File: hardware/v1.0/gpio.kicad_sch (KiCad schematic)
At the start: 23 parts, among them J2 HDMI_C_1.3, U1 ECP5U_12_CABGA256, U5 PCA9306DC1

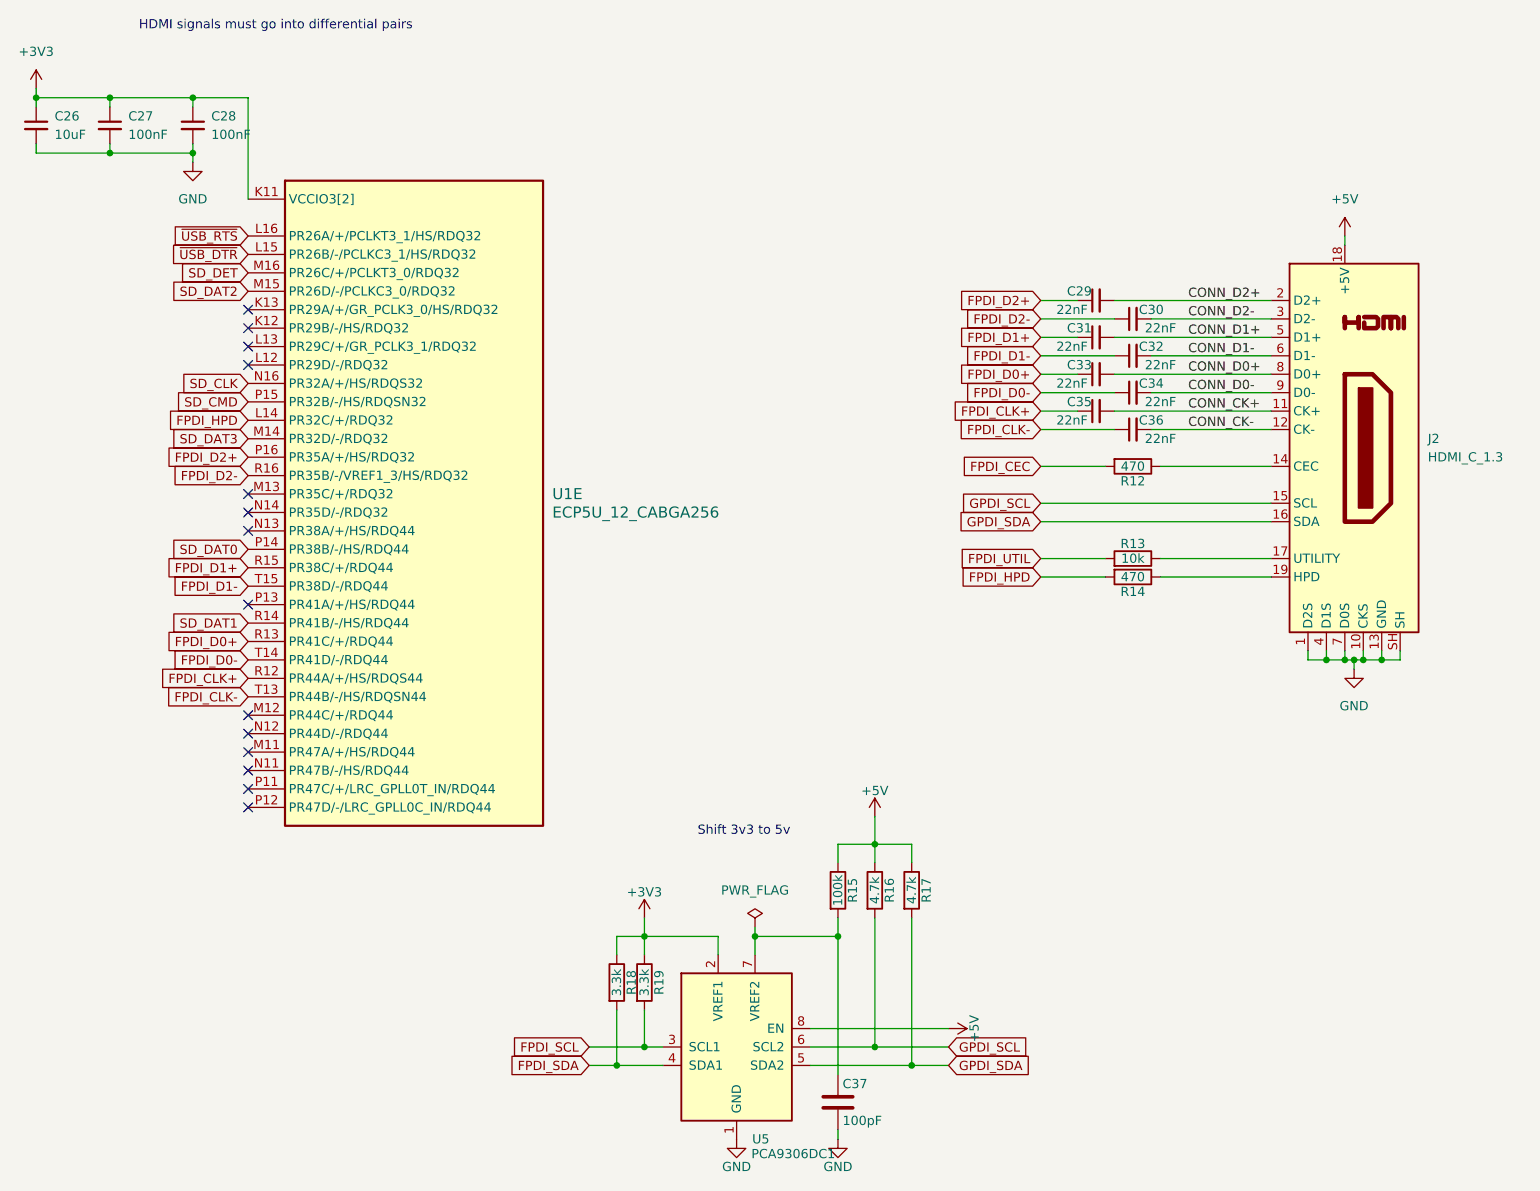
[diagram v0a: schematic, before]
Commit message: Forgot to commit yesterday
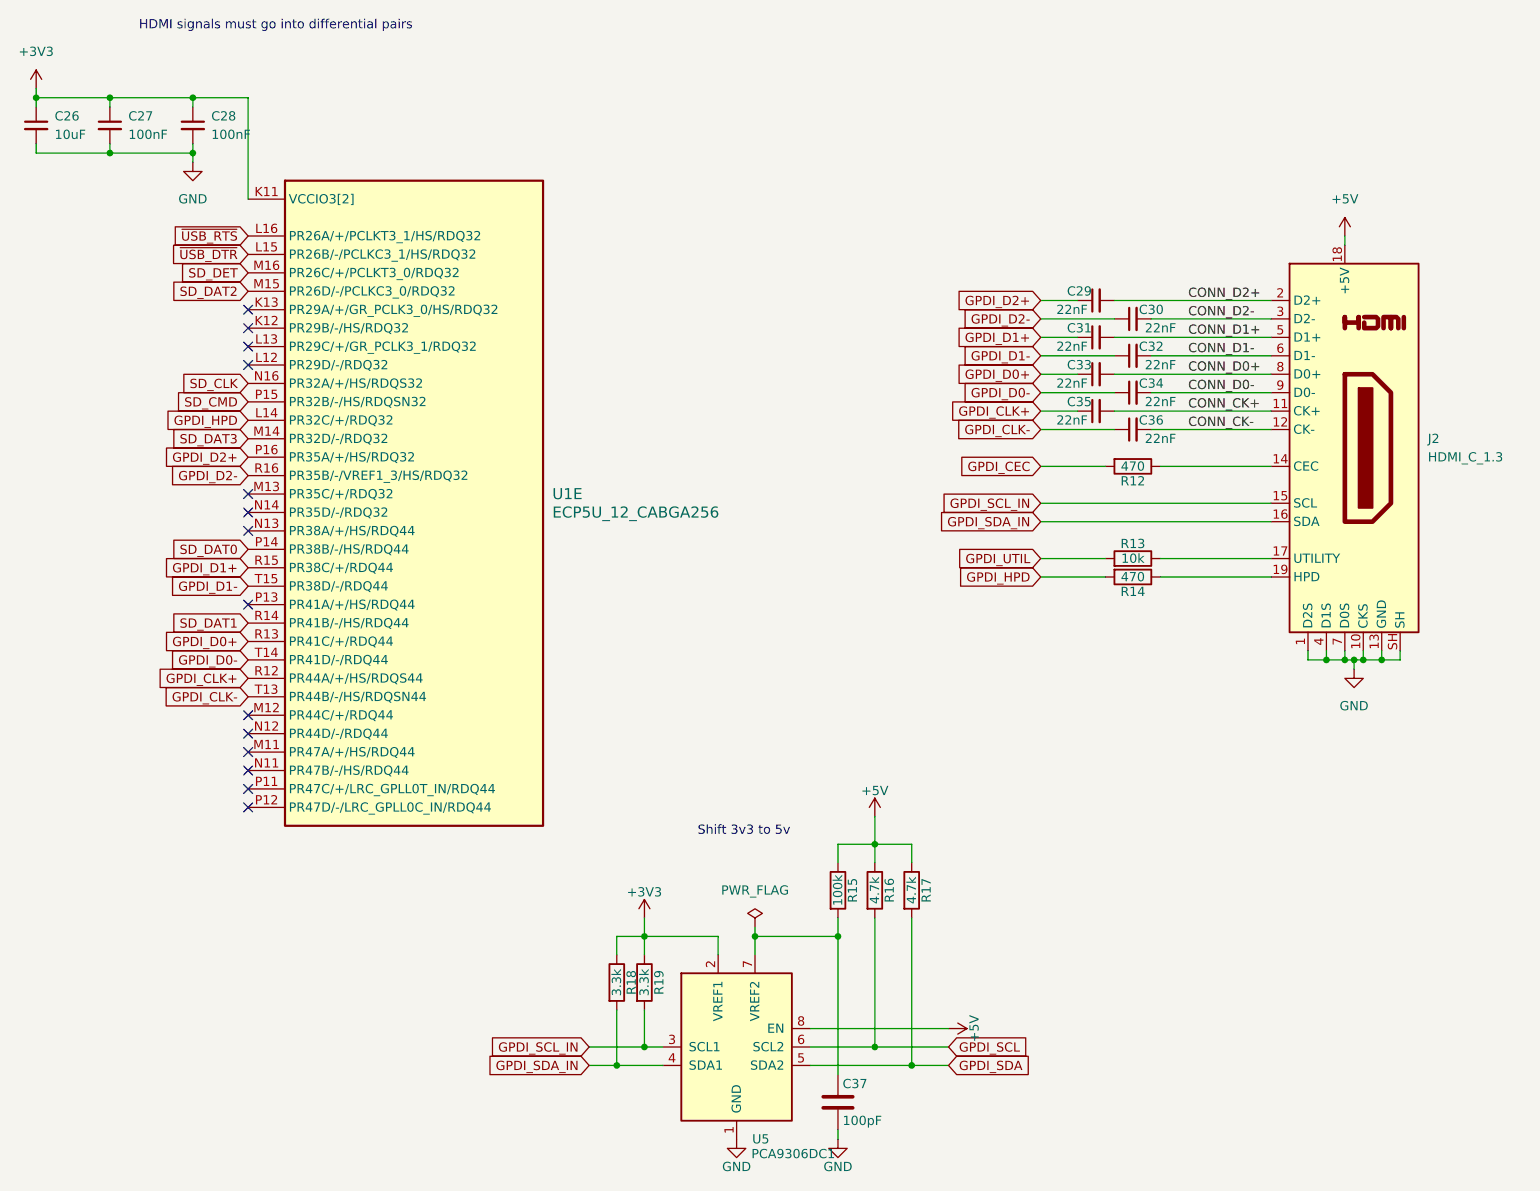
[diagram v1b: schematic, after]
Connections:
- net GPDI_SCL: no longer J2.15 (SCL)
- net GPDI_SDA: no longer J2.16 (SDA)
- net FPDI_CEC renamed GPDI_CEC
- net FPDI_CLK+ renamed GPDI_CLK+
- net FPDI_CLK- renamed GPDI_CLK-
- net FPDI_D0+ renamed GPDI_D0+
- net FPDI_D0- renamed GPDI_D0-
- net FPDI_D1+ renamed GPDI_D1+
- net FPDI_D1- renamed GPDI_D1-
- net FPDI_D2+ renamed GPDI_D2+
- net FPDI_D2- renamed GPDI_D2-
- net FPDI_HPD renamed GPDI_HPD
- net FPDI_SCL renamed GPDI_SCL_IN
- net GPDI_SCL_IN: now also J2.15 (SCL)
- net FPDI_SDA renamed GPDI_SDA_IN
- net GPDI_SDA_IN: now also J2.16 (SDA)
- net FPDI_UTIL renamed GPDI_UTIL
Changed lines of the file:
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@@
 		)
 	)
-	(global_label "FPDI_D2-"
+	(global_label "GPDI_D2-"
 		(shape input)
 		(at 171.45 73.66 180)
@@
 		)
 	)
-	(global_label "FPDI_CEC"
+	(global_label "GPDI_CEC"
 		(shape input)
 		(at 171.45 93.98 180)
@@
 		)
 	)
-	(global_label "FPDI_D2+"
+	(global_label "GPDI_D2+"
 		(shape input)
 		(at 62.23 92.71 180)
@@
 		)
 		(property "Intersheetrefs" "${INTERSHEET_REFS}"
-			(at 49.9919 92.71 0)
+			(at 49.8105 92.71 0)
 			(effects
 				(font
@@
 		)
 	)
-	(global_label "FPDI_CLK-"
+	(global_label "GPDI_CLK-"
 		(shape input)
 		(at 62.23 125.73 180)
@@
 		)
 		(property "Intersheetrefs" "${INTERSHEET_REFS}"
-			(at 48.9033 125.73 0)
-			(effects
-				(font
-					(size 1.27 1.27)
-				)
-				(justify right)
-				(hide yes)
-			)
-		)
-	)
-	(global_label "FPDI_CLK+"
+			(at 48.7219 125.73 0)
+			(effects
+				(font
+					(size 1.27 1.27)
+				)
+				(justify right)
+				(hide yes)
+			)
+		)
+	)
+	(global_label "GPDI_CLK+"
 		(shape input)
 		(at 171.45 86.36 180)
@@
 		)
 	)
-	(global_label "FPDI_UTIL"
+	(global_label "GPDI_UTIL"
 		(shape input)
 		(at 171.45 106.68 180)
@@
 		)
 	)
-	(global_label "FPDI_D1+"
+	(global_label "GPDI_D1+"
 		(shape input)
 		(at 62.23 107.95 180)
@@
 		)
 		(property "Intersheetrefs" "${INTERSHEET_REFS}"
-			(at 49.9919 107.95 0)
-			(effects
-				(font
-					(size 1.27 1.27)
-				)
-				(justify right)
-				(hide yes)
-			)
-		)
-	)
-	(global_label "FPDI_D1-"
+			(at 49.8105 107.95 0)
+			(effects
+				(font
+					(size 1.27 1.27)
+				)
+				(justify right)
+				(hide yes)
+			)
+		)
+	)
+	(global_label "GPDI_D1-"
 		(shape input)
 		(at 171.45 78.74 180)
@@
 		)
 	)
-	(global_label "FPDI_CLK-"
+	(global_label "GPDI_CLK-"
 		(shape input)
 		(at 171.45 88.9 180)
@@
 		)
 	)
-	(global_label "FPDI_HPD"
+	(global_label "GPDI_HPD"
 		(shape input)
 		(at 62.23 87.63 180)
@@
 		)
 		(property "Intersheetrefs" "${INTERSHEET_REFS}"
-			(at 50.1733 87.63 0)
-			(effects
-				(font
-					(size 1.27 1.27)
-				)
-				(justify right)
-				(hide yes)
-			)
-		)
-	)
-	(global_label "FPDI_D2-"
+			(at 49.9919 87.63 0)
+			(effects
+				(font
+					(size 1.27 1.27)
+				)
+				(justify right)
+				(hide yes)
+			)
+		)
+	)
+	(global_label "GPDI_D2-"
 		(shape input)
 		(at 62.23 95.25 180)
@@
 		)
 		(property "Intersheetrefs" "${INTERSHEET_REFS}"
-			(at 49.9919 95.25 0)
+			(at 49.8105 95.25 0)
 			(effects
 				(font
@@
 		)
 	)
-	(global_label "FPDI_SDA"
+	(global_label "GPDI_SDA_IN"
 		(shape input)
 		(at 109.22 176.53 180)
@@
 		)
 	)
-	(global_label "FPDI_SCL"
+	(global_label "GPDI_SCL_IN"
 		(shape input)
 		(at 109.22 173.99 180)
@@
 		)
 	)
-	(global_label "FPDI_HPD"
+	(global_label "GPDI_HPD"
 		(shape input)
 		(at 171.45 109.22 180)
@@
 		)
 	)
-	(global_label "FPDI_D1+"
+	(global_label "GPDI_D1+"
 		(shape input)
 		(at 171.45 76.2 180)
@@
 		)
 	)
-	(global_label "FPDI_D1-"
+	(global_label "GPDI_D1-"
 		(shape input)
 		(at 62.23 110.49 180)
@@
 		)
 		(property "Intersheetrefs" "${INTERSHEET_REFS}"
-			(at 49.9919 110.49 0)
-			(effects
-				(font
-					(size 1.27 1.27)
-				)
-				(justify right)
-				(hide yes)
-			)
-		)
-	)
-	(global_label "GPDI_SDA"
+			(at 49.8105 110.49 0)
+			(effects
+				(font
+					(size 1.27 1.27)
+				)
+				(justify right)
+				(hide yes)
+			)
+		)
+	)
+	(global_label "GPDI_SDA_IN"
 		(shape input)
 		(at 171.45 101.6 180)
@@
 		)
 	)
-	(global_label "FPDI_CLK+"
+	(global_label "GPDI_CLK+"
 		(shape input)
 		(at 62.23 123.19 180)
@@
 		)
 		(property "Intersheetrefs" "${INTERSHEET_REFS}"
-			(at 48.9033 123.19 0)
+			(at 48.7219 123.19 0)
 			(effects
 				(font
@@
 		)
 	)
-	(global_label "FPDI_D0+"
+	(global_label "GPDI_D0+"
 		(shape input)
 		(at 171.45 81.28 180)
@@
 		)
 	)
-	(global_label "GPDI_SCL"
+	(global_label "GPDI_SCL_IN"
 		(shape input)
 		(at 171.45 99.06 180)
@@
 		)
 	)
-	(global_label "FPDI_D2+"
+	(global_label "GPDI_D2+"
 		(shape input)
 		(at 171.45 71.12 180)
@@
 		)
 	)
-	(global_label "FPDI_D0-"
+	(global_label "GPDI_D0-"
 		(shape input)
 		(at 62.23 120.65 180)
@@
 		)
 		(property "Intersheetrefs" "${INTERSHEET_REFS}"
-			(at 49.9919 120.65 0)
-			(effects
-				(font
-					(size 1.27 1.27)
-				)
-				(justify right)
-				(hide yes)
-			)
-		)
-	)
-	(global_label "FPDI_D0+"
+			(at 49.8105 120.65 0)
+			(effects
+				(font
+					(size 1.27 1.27)
+				)
+				(justify right)
+				(hide yes)
+			)
+		)
+	)
+	(global_label "GPDI_D0+"
 		(shape input)
 		(at 62.23 118.11 180)
@@
 		)
 		(property "Intersheetrefs" "${INTERSHEET_REFS}"
-			(at 49.9919 118.11 0)
-			(effects
-				(font
-					(size 1.27 1.27)
-				)
-				(justify right)
-				(hide yes)
-			)
-		)
-	)
-	(global_label "FPDI_D0-"
+			(at 49.8105 118.11 0)
+			(effects
+				(font
+					(size 1.27 1.27)
+				)
+				(justify right)
+				(hide yes)
+			)
+		)
+	)
+	(global_label "GPDI_D0-"
 		(shape input)
 		(at 171.45 83.82 180)
